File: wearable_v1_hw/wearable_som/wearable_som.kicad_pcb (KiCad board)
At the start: 2 copper layers, 40 x 30 mm, 39 parts, among them IC1 TPS7A0228PDBVR, IC2 DA7280-00FV2, J1 Conn_01x04, J2 USB4105-GF-A, M1 Motor_DC, Q1 PMOS, SW1 Reset, SW2 SW_Nidec_CAS-120A1, SW3 Boot, U1 STM32WB55RGVx, U2 BMI270, U3 MCP73831-2-MC, U4 DLF162500LT-5028A1, U5 2450AT18A100E, U6 USBLC6-2SC6, Y1 Crystal_GND23

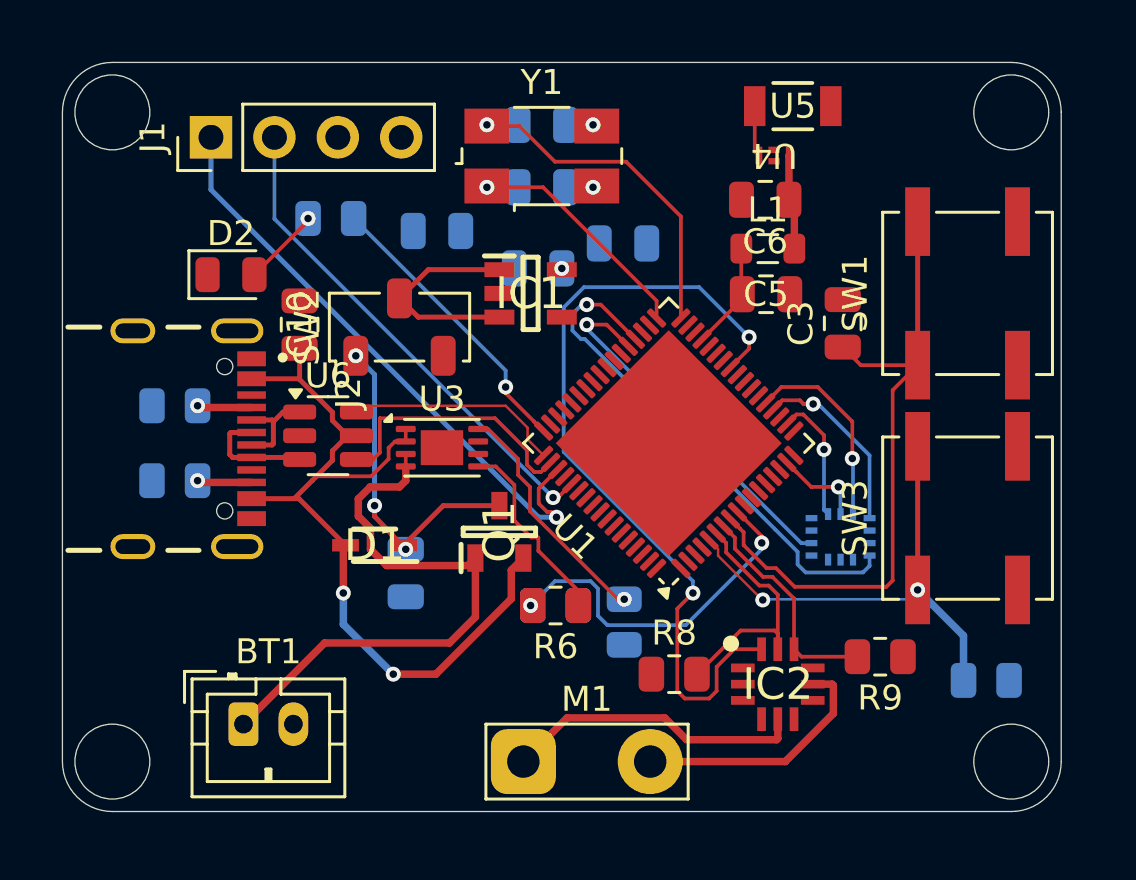
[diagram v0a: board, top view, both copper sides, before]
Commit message: init layout done
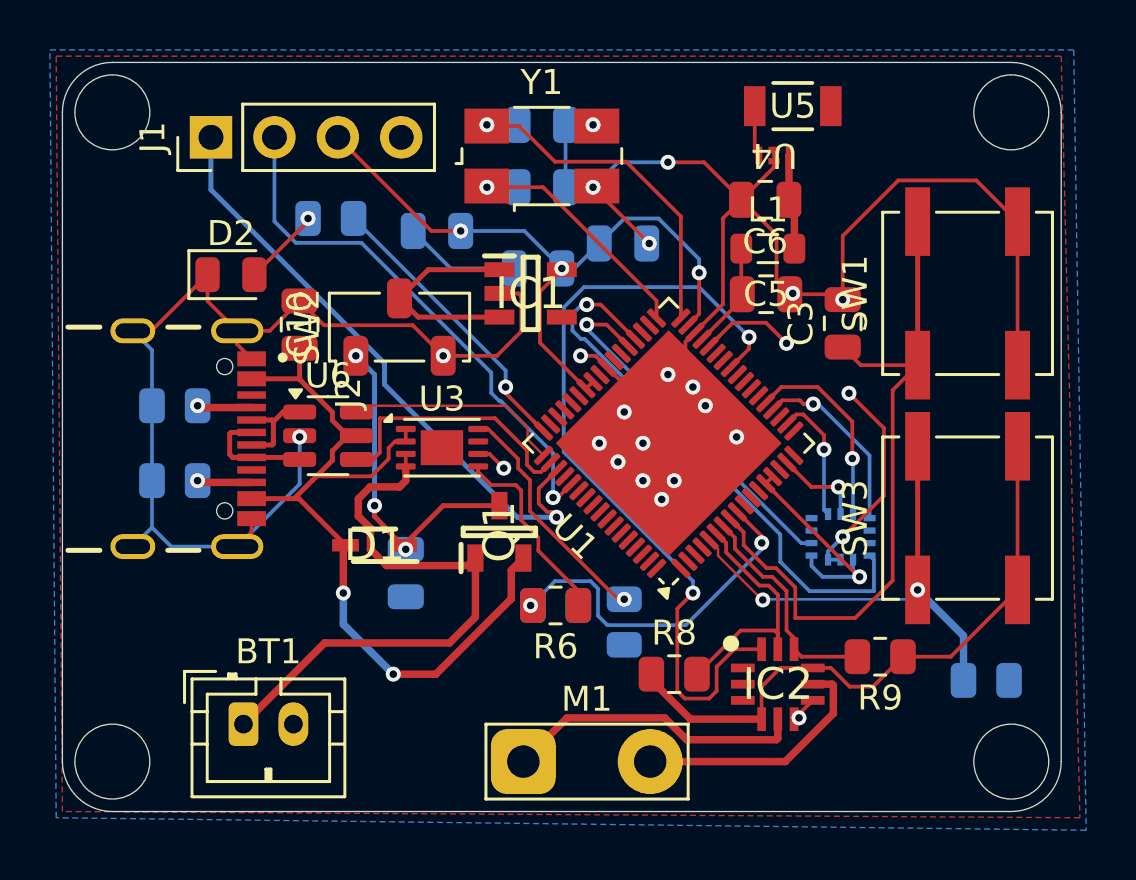
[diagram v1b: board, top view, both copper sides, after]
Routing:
- net GND: track 2.20 -> 116.8 mm, vias 2 -> 24
- net +3.3V: track 0.00 -> 65.0 mm, vias 1 -> 5
- net /INT1: track 20.6 -> 22.5 mm
- net /NRST: track 26.1 -> 27.9 mm
- net /SWCLK: track 20.0 -> 21.6 mm
- net /SWDIO: track 24.0 -> 24.5 mm
- added copper zone on F.Cu, net +3.3V
- added copper zone on B.Cu, net GND
